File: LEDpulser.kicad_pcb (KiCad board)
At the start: 2 copper layers, 59 parts, among them J1 RJ45_Shielded, J2 0731375003, J3 0731375003, J4 Conn_01x04_Female, Q1 AO3401A, Q2 AO3400A, Q3 AO3400A, SW1 ATE1D-5M3-10-Z, U1 74HC123, U10 LT3082, U2 74HC123, U3 74HC123, U4 74HC10, U5 LT1121-5, U6 PM8834, U7 NE555, U8 PM8834, U9 PM8834

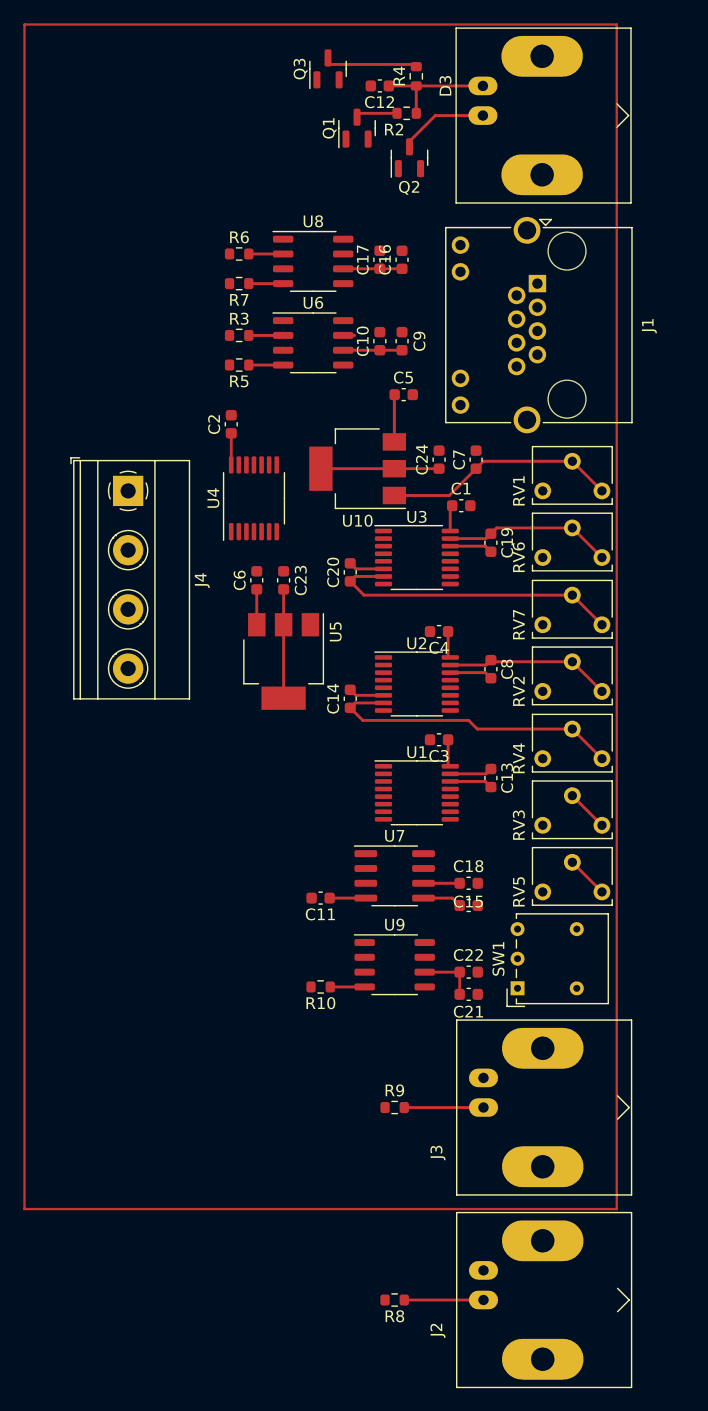
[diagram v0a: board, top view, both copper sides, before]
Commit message: Routed first draft
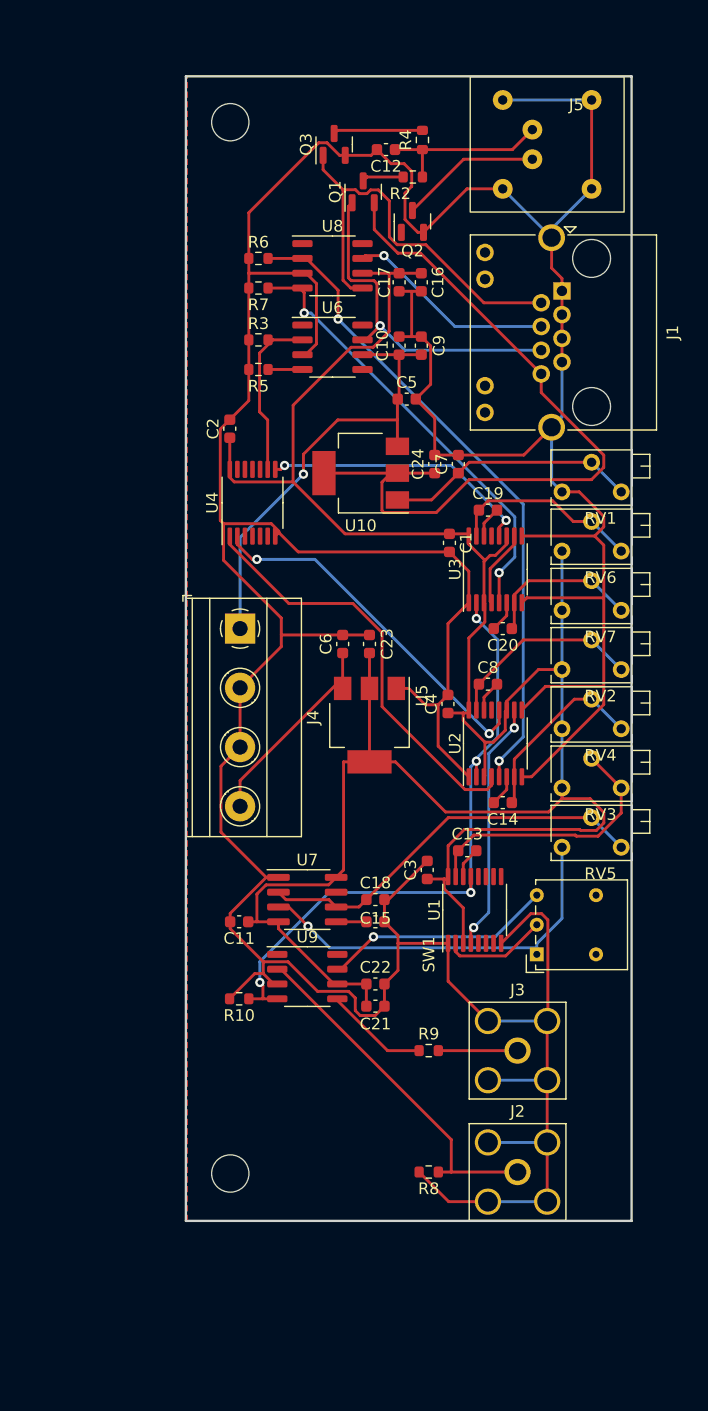
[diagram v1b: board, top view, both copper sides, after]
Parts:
- removed D3: LED, Connector_Coaxial:BNC_Amphenol_B6252HB-NPP3G-50_Horizontal
- added H1: MountingHole, MountingHole:MountingHole_3.2mm_M3, F.Cu at (105.3, 29.3)
- added H2: MountingHole, MountingHole:MountingHole_3.2mm_M3, F.Cu at (105.3, 119.5)
- added J5: LED, Connector:FanPinHeader_1x03_P2.54mm_Vertical, F.Cu at (132.5, 31.2)
- C13: value 330pF -> C
- J2, J3: value 0731375003 -> EPS.00.250.NTN; footprint Connector_Coaxial:BNC_Amphenol_B6252HB-NPP3G-50_Horizontal -> Connector_Coaxial:SMA_Amphenol_132203-12_Horizontal
- R4: value 100 -> 50
- RV1: footprint Potentiometer_THT:Potentiometer_Vishay_T73XX_Horizontal -> Potentiometer_THT:Potentiometer_Bourns_3266X_Horizontal
- RV2, RV3, RV4, RV6, RV7: value 1k -> 2k; footprint Potentiometer_THT:Potentiometer_Vishay_T73XX_Horizontal -> Potentiometer_THT:Potentiometer_Bourns_3266X_Horizontal
- RV5: value 1k -> 1M; footprint Potentiometer_THT:Potentiometer_Vishay_T73XX_Horizontal -> Potentiometer_THT:Potentiometer_Bourns_3266X_Horizontal
- moved C14 15.8 mm to (128.7, 87.7), turned to 180 degrees
- moved J4 15.2 mm to (106.1, 72.8)
- moved C20 13.9 mm to (128.7, 72.8), turned to 180 degrees
- moved R8 11.4 mm to (122.3, 119.4)
- moved J2 11.4 mm to (129.9, 119.4)
- moved C3 11.2 mm to (122.2, 93.5), turned to 90 degrees
- moved U1 11.2 mm to (126.2, 96.9), turned to 90 degrees
- moved C23 9.17 mm to (117.2, 74.1)
- moved C6 9.17 mm to (114.9, 74.1)
- moved U5 9.17 mm to (117.2, 81.1)
- moved U2 8.44 mm to (128.0, 82.6), turned to 90 degrees
- moved C15 8.12 mm to (117.7, 97.9)
- moved C18 8.12 mm to (117.7, 96.0)
- moved C21 8.07 mm to (117.7, 105.2)
- moved C22 8.07 mm to (117.7, 103.3)
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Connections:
- Q2 pad 1: /LED_ON -> unconnected-(Q2-Pad1)
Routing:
- net GND: track 0.00 -> 410.9 mm
- net +5V: track 32.2 -> 207.9 mm
- net /CAP_VOLTAGE: track 10.1 -> 65.7 mm
- net Net-(R6-Pad1): track 2.95 -> 56.3 mm, vias 0 -> 2
- net Net-(R10-Pad1): track 2.95 -> 55.6 mm, vias 0 -> 4
- net Net-(U2-Pad4): track 0.00 -> 36.5 mm
- net /LED_SHORT: track 0.00 -> 36.5 mm
- net Net-(R7-Pad1): track 2.95 -> 38.5 mm, vias 0 -> 2
- net /INT: track 0.00 -> 33.7 mm, vias 0 -> 1
- net Net-(U2-Pad12): track 0.00 -> 31.4 mm, vias 0 -> 2
- net +12V: track 9.11 -> 39.5 mm, vias 0 -> 1
- net /CAP_CHARGE: track 0.99 -> 29.7 mm, vias 0 -> 1
- net Net-(C18-Pad1): track 6.69 -> 34.2 mm
- net /EXT: track 6.80 -> 30.6 mm
- net Net-(U3-Pad12): track 0.00 -> 23.5 mm, vias 0 -> 2
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- added copper zone on B.Cu, net GND
- added copper zone on F.Cu, net GND
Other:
- board outline added: 38.2 x 98.2 mm
